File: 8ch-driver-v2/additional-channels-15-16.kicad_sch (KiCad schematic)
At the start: 28 parts, among them Q15 2N7002E, Q16 2N7002E, U15 DRV104PWP, U16 DRV104PWP

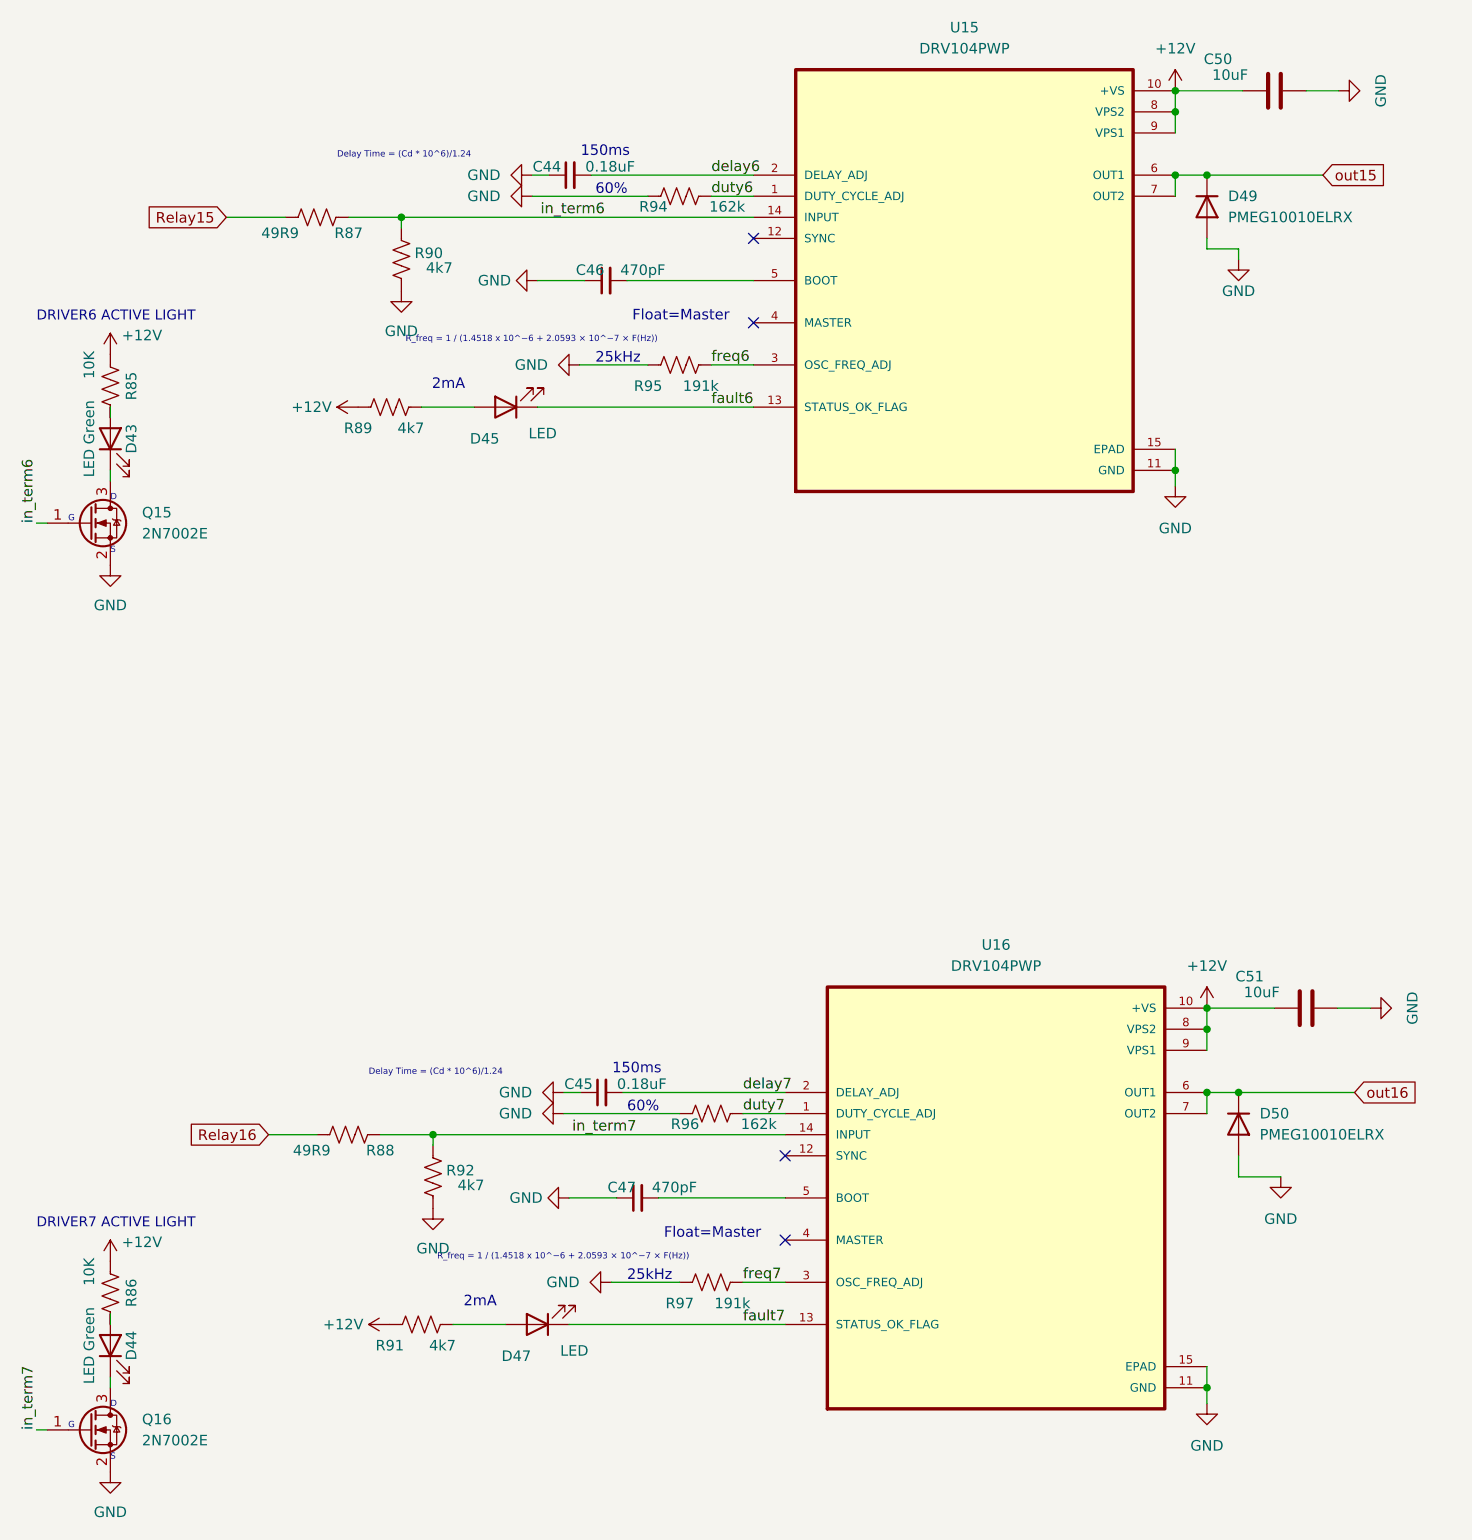
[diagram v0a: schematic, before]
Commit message: mucho mas progresso
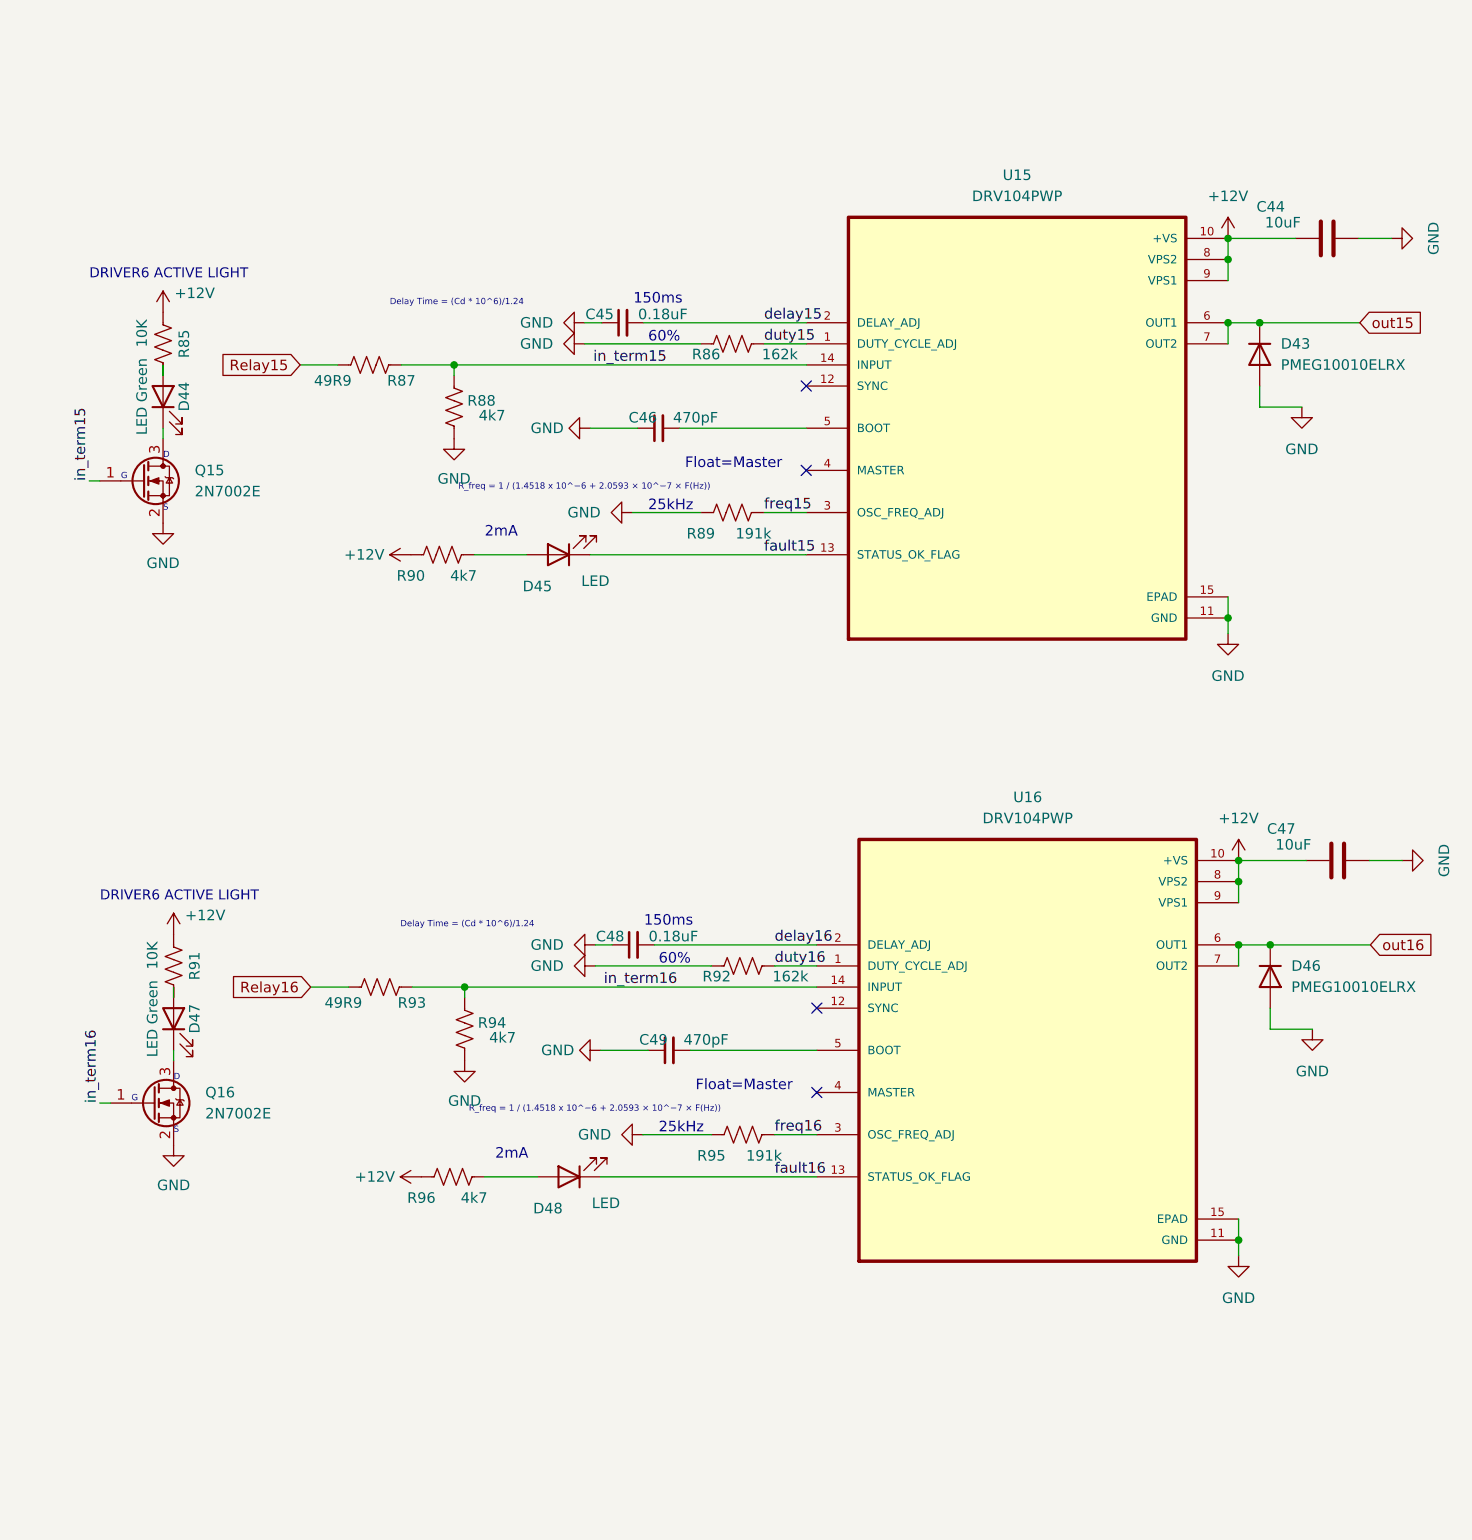
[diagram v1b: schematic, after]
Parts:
- removed C44: 0.18uF, Capacitor_SMD:C_1206_3216Metric, symbol Device:C_Small
- removed C47: 470pF, Capacitor_SMD:C_1206_3216Metric, symbol Device:C_Small
- removed C50, C51: 10uF, Capacitor_SMD:C_1210_3225Metric, symbol Device:C
- removed D43: LED Green, LED_SMD:LED_0805_2012Metric, symbol Device:LED
- removed D49, D50: PMEG10010ELRX, Diode_SMD:Nexperia_CFP3_SOD-123W, symbol Device:D
- removed R97: 191k, Resistor_SMD:R_1206_3216Metric, symbol Device:R_US
- added C44, C47: 10uF, Capacitor_SMD:C_1210_3225Metric, symbol Device:C
- added C48: 0.18uF, Capacitor_SMD:C_1206_3216Metric, symbol Device:C_Small
- added C49: 470pF, Capacitor_SMD:C_1206_3216Metric, symbol Device:C_Small
- added D43, D46: PMEG10010ELRX, Diode_SMD:Nexperia_CFP3_SOD-123W, symbol Device:D
- added D48: LED, LED_SMD:LED_0805_2012Metric, symbol Device:LED
- added R93: 49R9, Resistor_SMD:R_1206_3216Metric, symbol Device:R_US
- D47: value LED -> LED Green
- R86: value 10K -> 162k
- R88: value 49R9 -> 4k7; PartNum RC0805FR-0749R9L -> RC0805JR-074K7L
- R89: value 4k7 -> 191k; PartNum RC0805JR-074K7L -> RC0805FR-07191KL
- R91: value 4k7 -> 10K; PartNum RC0805JR-074K7L -> RC0805FR-07162KL
- R92: value 4k7 -> 162k; PartNum RC0805JR-074K7L -> RC0805FR-07162KL
- R94, R96: value 162k -> 4k7; PartNum RC0805FR-07162KL -> RC0805JR-074K7L
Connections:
- net +12V: now also R90.1, R96.1, C44.1, C47.1; no longer R86.1, R89.1
- net GND: now also R86.1, R88.1, R89.1, C44.2, C47.2, C48.1, C49.1, D43.2 (A), D46.2 (A); no longer R90.1, R96.1
- net Relay16: now also R93.1; no longer R88.1
- net out15: now also D43.1 (K)
- net out16: now also D46.1 (K)
- net at Q15.3 (D): now also D44.1 (K)
- net at D45.2 (A): now also R90.2; no longer R89.2
- net at U16.5 (BOOT): now also C49.2
- net at R85.2: now also D44.2 (A)
- net at Q16.3 (D): now also D47.1 (K); no longer D44.1 (K)
- net duty15: now reaches R86.2
- net duty15: now also U15.1 (DUTY_CYCLE_ADJ); no longer D44.2 (A)
- net delay6 renamed delay15
- net delay15: now also C45.2
- net delay7 renamed delay16
- net delay16: now also C48.2; no longer C45.2
- net duty6 renamed in_term16
- net in_term16: now also Q16.1 (G), U16.14 (INPUT), R93.2; no longer U15.1 (DUTY_CYCLE_ADJ)
- net duty7: no longer names the net of R96.2
- net duty7: now also D48.2 (A); no longer U16.1 (DUTY_CYCLE_ADJ)
- net fault6 renamed fault15
- net fault7 renamed fault16
- net fault16: now also D48.1 (K); no longer D47.1 (K)
- net freq6 renamed freq15
- net freq15: now also R89.2; no longer R95.2
- net freq7 renamed freq16
- net freq16: now also R95.2
- net in_term6 renamed in_term15
- net in_term15: now also R88.2; no longer R90.2
- removed net in_term7: Q16.1 (G), R88.2, R92.2, U16.14 (INPUT)
- new net duty16: R92.2, U16.1 (DUTY_CYCLE_ADJ)
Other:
- note removed: "DRIVER7 ACTIVE LIGHT"
